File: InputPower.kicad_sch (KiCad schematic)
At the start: 34 parts, among them IC3 RT8293BHZSP, IC4 RT8293BHZSP

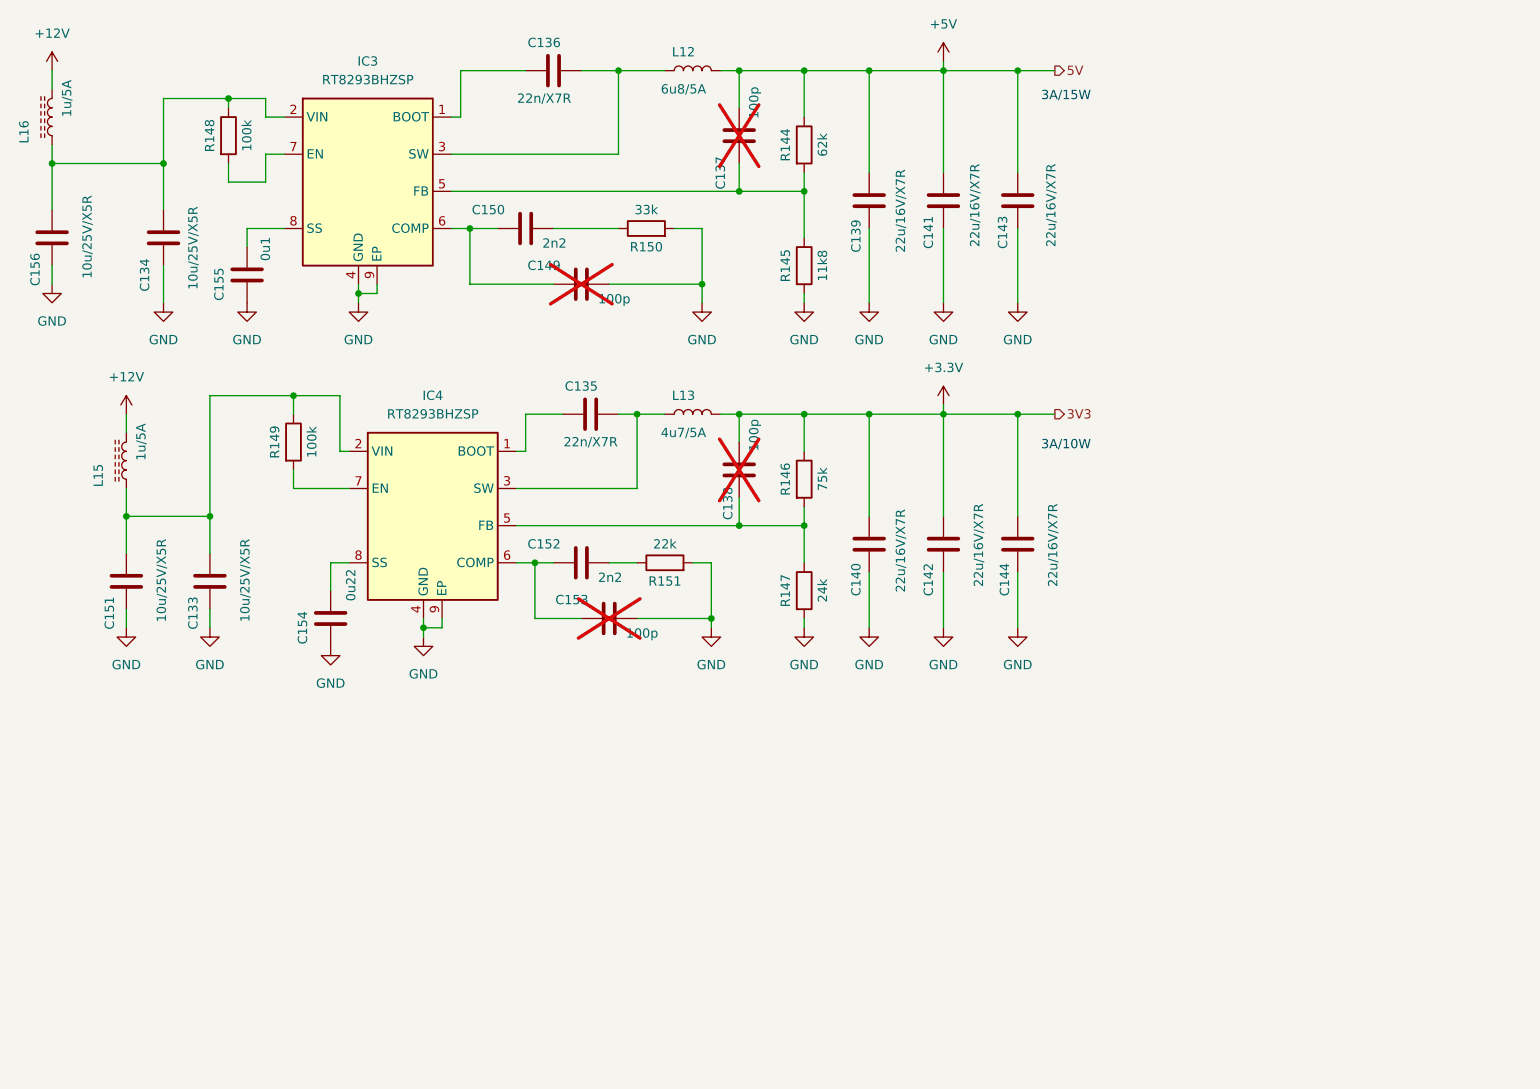
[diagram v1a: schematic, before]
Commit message: IMU block implementation
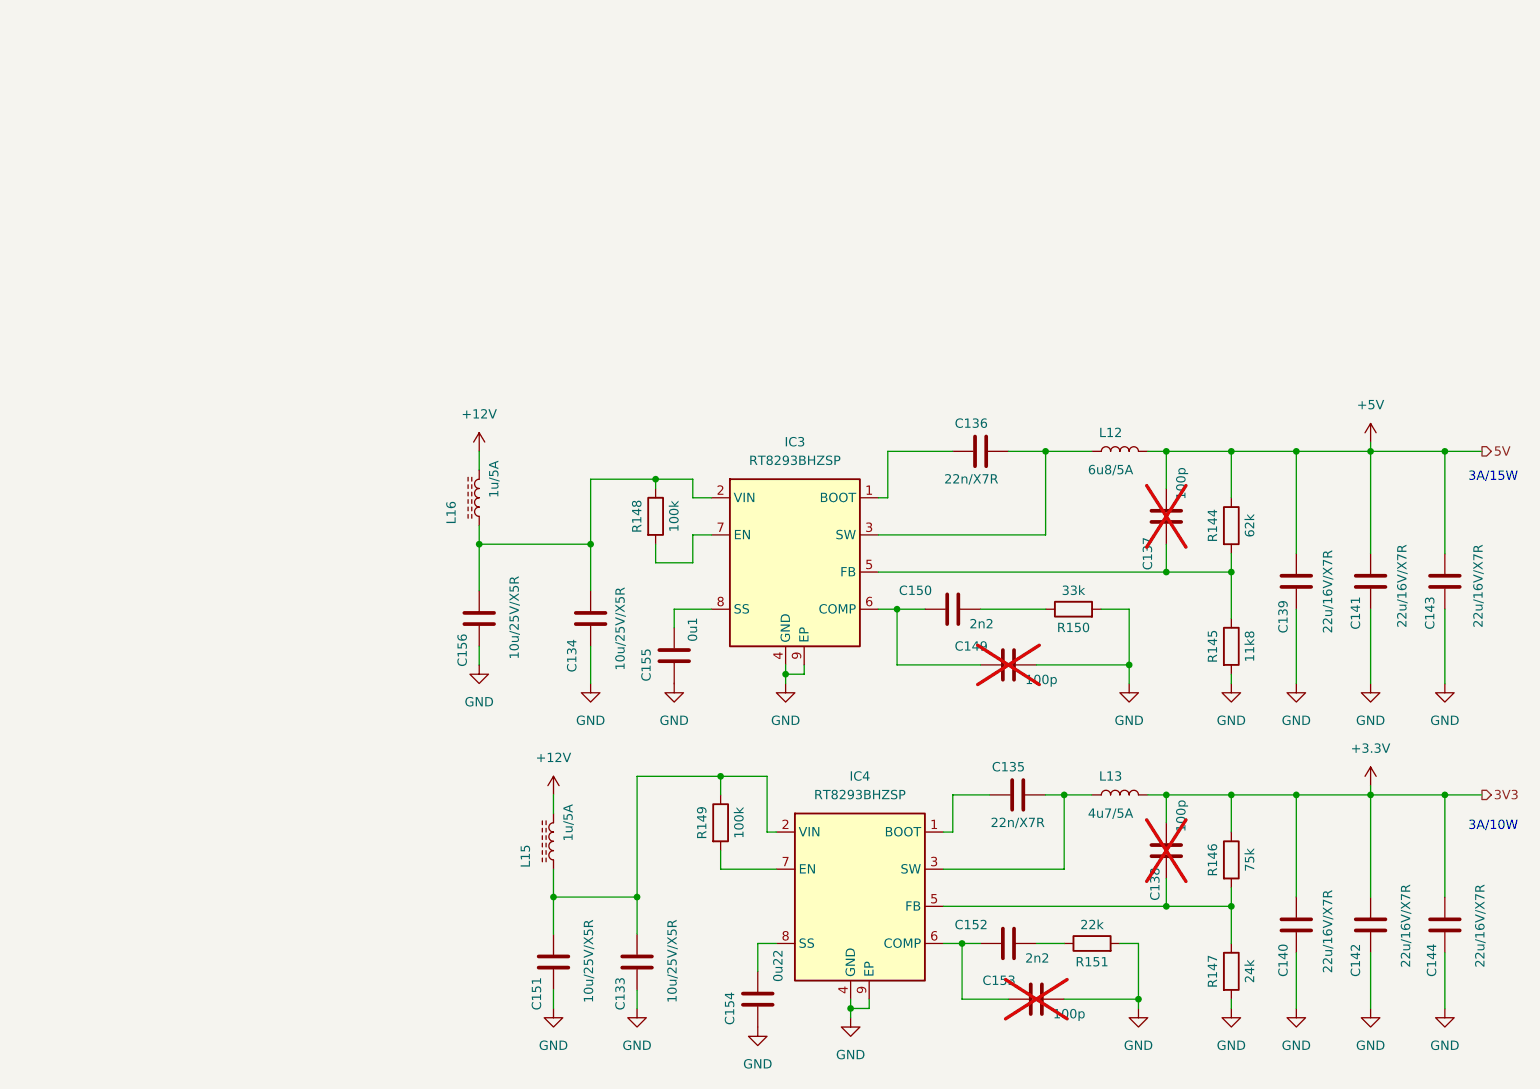
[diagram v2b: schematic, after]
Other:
- moved on the sheet: C133, C134, C135, C136, C137, C138, C139, C140, C141, C142, C143, C144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
